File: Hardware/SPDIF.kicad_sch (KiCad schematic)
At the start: 8 parts, among them J10 Conn_Coaxial, J9 Conn_Coaxial, T1 DA100J

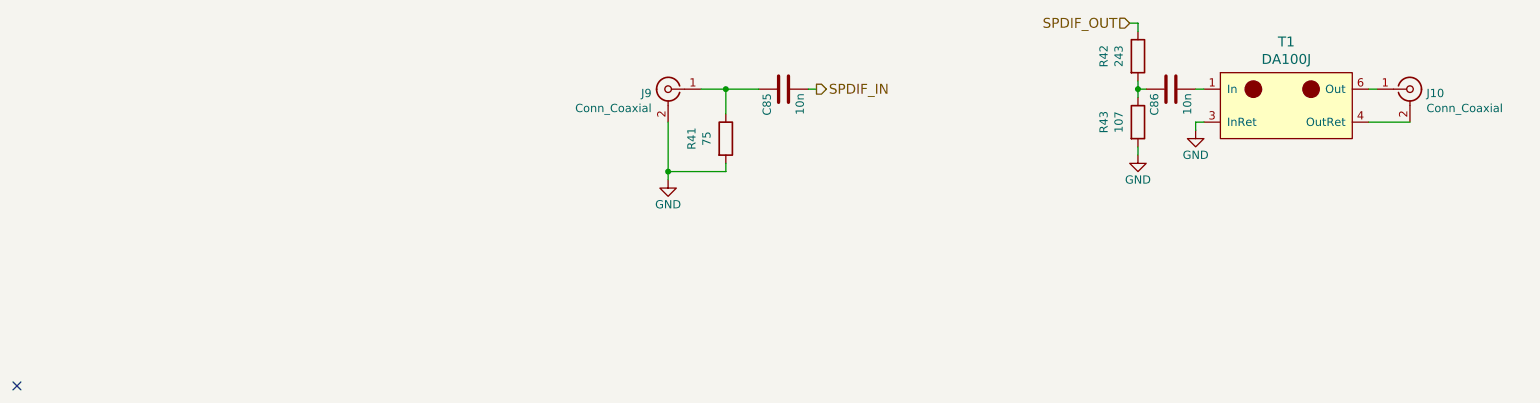
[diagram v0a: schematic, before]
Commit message: Updated power supply
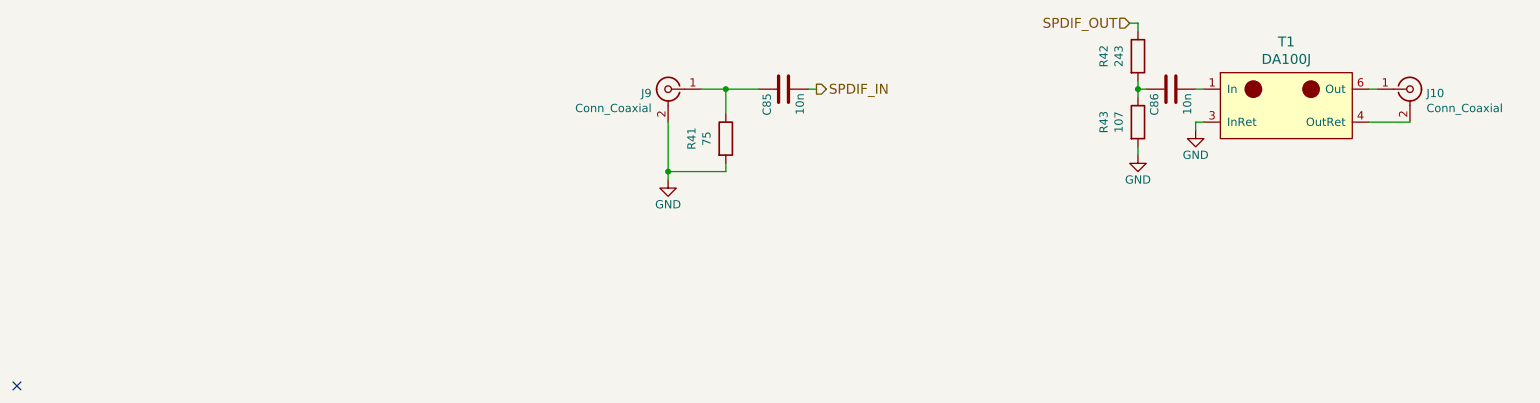
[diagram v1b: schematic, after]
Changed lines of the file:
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@@
     (pin "2")
   )
-  (symbol (lib_id "Device:R") (at 97.79 96.52 0)
+  (symbol (lib_id "Device:R") (at 97.79 96.52 0) (unit 1)
     (in_bom yes) (on_board yes)
     (property "Reference" "R41" (id 0) (at 92.5322 96.52 90))
@@
     (pin "2")
   )
-  (symbol (lib_id "Device:R") (at 161.29 93.98 0)
+  (symbol (lib_id "Device:R") (at 161.29 93.98 0) (unit 1)
     (in_bom yes) (on_board yes)
     (property "Reference" "R43" (id 0) (at 156.0322 93.98 90))
@@
     (pin "2")
   )
-  (symbol (lib_id "Device:R") (at 161.29 83.82 0)
+  (symbol (lib_id "Device:R") (at 161.29 83.82 0) (unit 1)
     (in_bom yes) (on_board yes)
     (property "Reference" "R42" (id 0) (at 156.0322 83.82 90))

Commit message: feat: updated amplifier IC, finalized design
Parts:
- C85, C86: footprint Capacitor_SMD:C_0603_1608Metric_Pad1.08x0.95mm_HandSolder -> Capacitor_SMD:C_0402_1005Metric
- R41, R42, R43: footprint Resistor_SMD:R_0603_1608Metric_Pad0.98x0.95mm_HandSolder -> Resistor_SMD:R_0402_1005Metric
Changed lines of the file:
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@@
       (effects (font (size 1.27 1.27)) (justify left))
     )
-    (property "Footprint" "Capacitor_SMD:C_0603_1608Metric_Pad1.08x0.95mm_HandSolder" (id 2) (at 110.49 89.8652 0)
+    (property "Footprint" "Capacitor_SMD:C_0402_1005Metric" (id 2) (at 110.49 89.8652 0)
       (effects (font (size 0.762 0.762)) hide)
     )
-    (property "Datasheet" "" (id 3) (at 106.68 88.9 0)
+    (property "Datasheet" "~" (id 3) (at 106.68 88.9 0)
       (effects (font (size 1.524 1.524)))
     )
@@
     (property "Reference" "R41" (id 0) (at 92.5322 96.52 90))
     (property "Value" "75" (id 1) (at 94.8436 96.52 90))
-    (property "Footprint" "Resistor_SMD:R_0603_1608Metric_Pad0.98x0.95mm_HandSolder" (id 2) (at 96.012 96.52 90)
+    (property "Footprint" "Resistor_SMD:R_0402_1005Metric" (id 2) (at 96.012 96.52 90)
       (effects (font (size 1.27 1.27)) hide)
     )
@@
       (effects (font (size 1.27 1.27)) (justify left))
     )
-    (property "Footprint" "Capacitor_SMD:C_0603_1608Metric_Pad1.08x0.95mm_HandSolder" (id 2) (at 170.18 89.8652 0)
+    (property "Footprint" "Capacitor_SMD:C_0402_1005Metric" (id 2) (at 170.18 89.8652 0)
       (effects (font (size 0.762 0.762)) hide)
     )
-    (property "Datasheet" "" (id 3) (at 166.37 88.9 0)
+    (property "Datasheet" "~" (id 3) (at 166.37 88.9 0)
       (effects (font (size 1.524 1.524)))
     )
@@
     (property "Reference" "R43" (id 0) (at 156.0322 93.98 90))
     (property "Value" "107" (id 1) (at 158.3436 93.98 90))
-    (property "Footprint" "Resistor_SMD:R_0603_1608Metric_Pad0.98x0.95mm_HandSolder" (id 2) (at 159.512 93.98 90)
+    (property "Footprint" "Resistor_SMD:R_0402_1005Metric" (id 2) (at 159.512 93.98 90)
       (effects (font (size 1.27 1.27)) hide)
     )
@@
     (property "Reference" "R42" (id 0) (at 156.0322 83.82 90))
     (property "Value" "243" (id 1) (at 158.3436 83.82 90))
-    (property "Footprint" "Resistor_SMD:R_0603_1608Metric_Pad0.98x0.95mm_HandSolder" (id 2) (at 159.512 83.82 90)
+    (property "Footprint" "Resistor_SMD:R_0402_1005Metric" (id 2) (at 159.512 83.82 90)
       (effects (font (size 1.27 1.27)) hide)
     )
